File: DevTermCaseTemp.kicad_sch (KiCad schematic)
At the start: 1 part, among them J1 miniPCIe

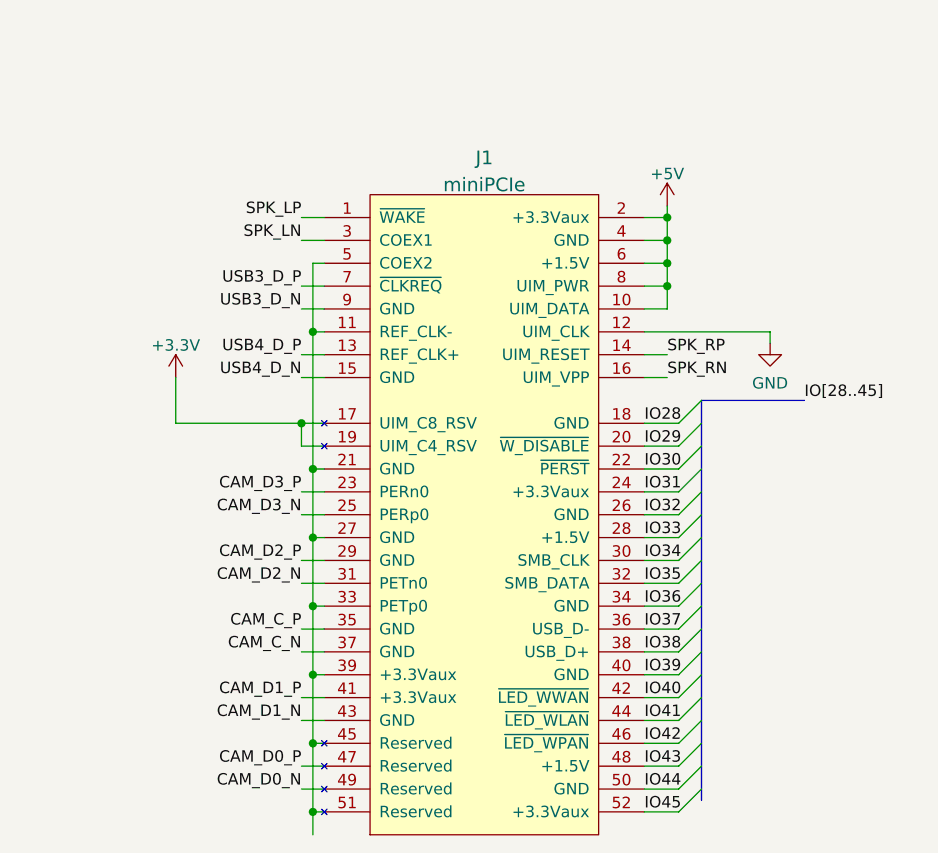
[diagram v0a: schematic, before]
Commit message: Update README
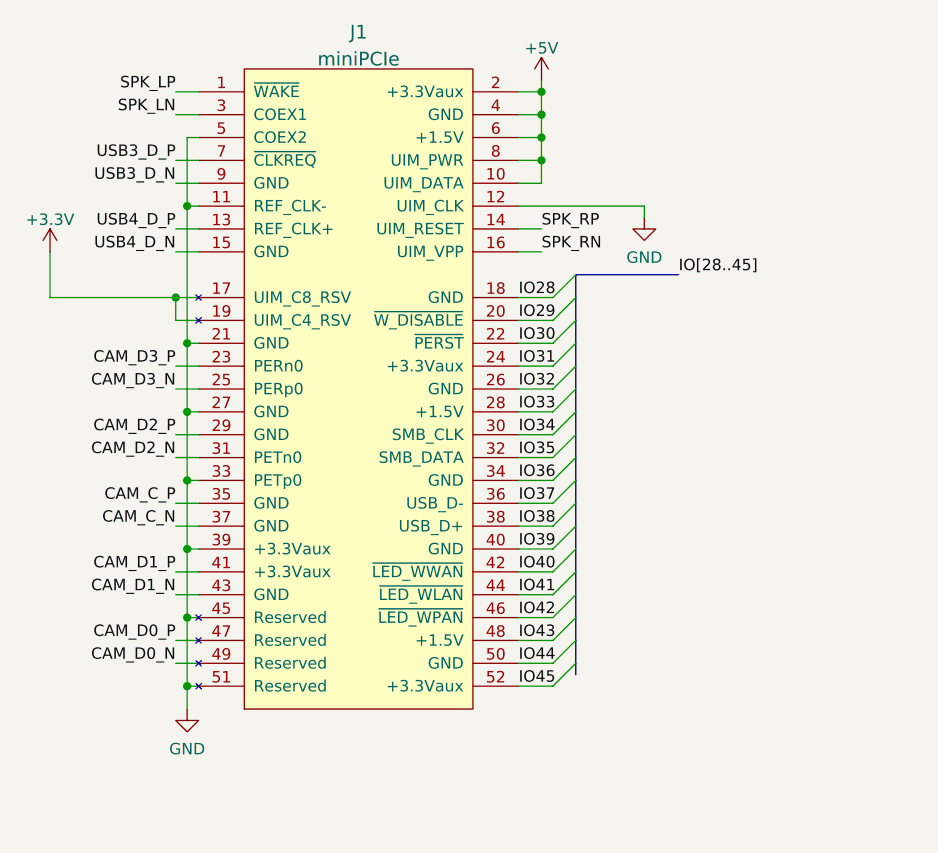
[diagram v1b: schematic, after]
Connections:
- net GND: now also J1.11 (REF_CLK-), J1.21 (GND), J1.27 (GND), J1.33 (PETp0), J1.39 (+3.3Vaux), J1.45 (Reserved), J1.5 (COEX2), J1.51 (Reserved)
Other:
- moved on the sheet: J1
